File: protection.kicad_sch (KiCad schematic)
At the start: 30 parts, among them J10 10x2.54mm, J5 10x2.54mm, J6 10x2.54mm, J7 10x2.54mm, J8 10x2.54mm, J9 10x2.54mm, K19 TQ2-5, U6 TXS0108EPW, U7 TXS0108EPW, U8 TXS0108EPW

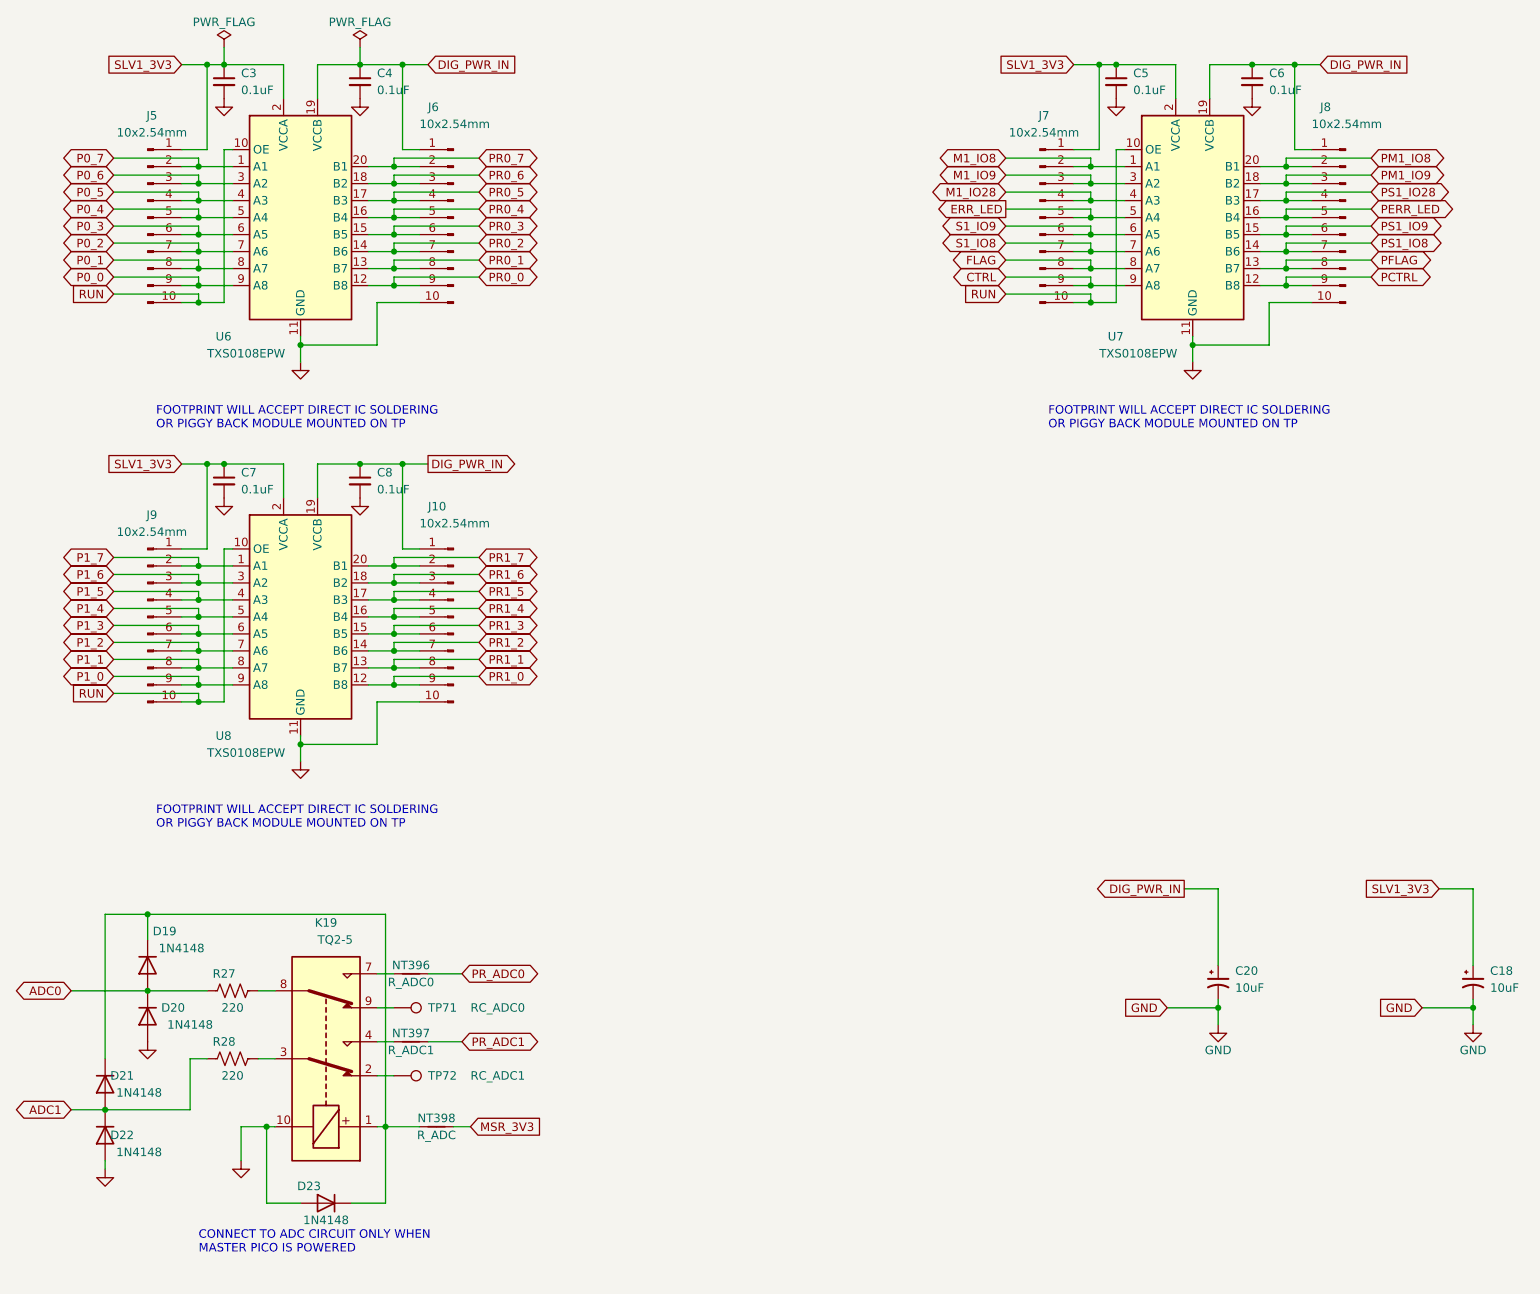
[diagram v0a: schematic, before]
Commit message: update
Correction of small error
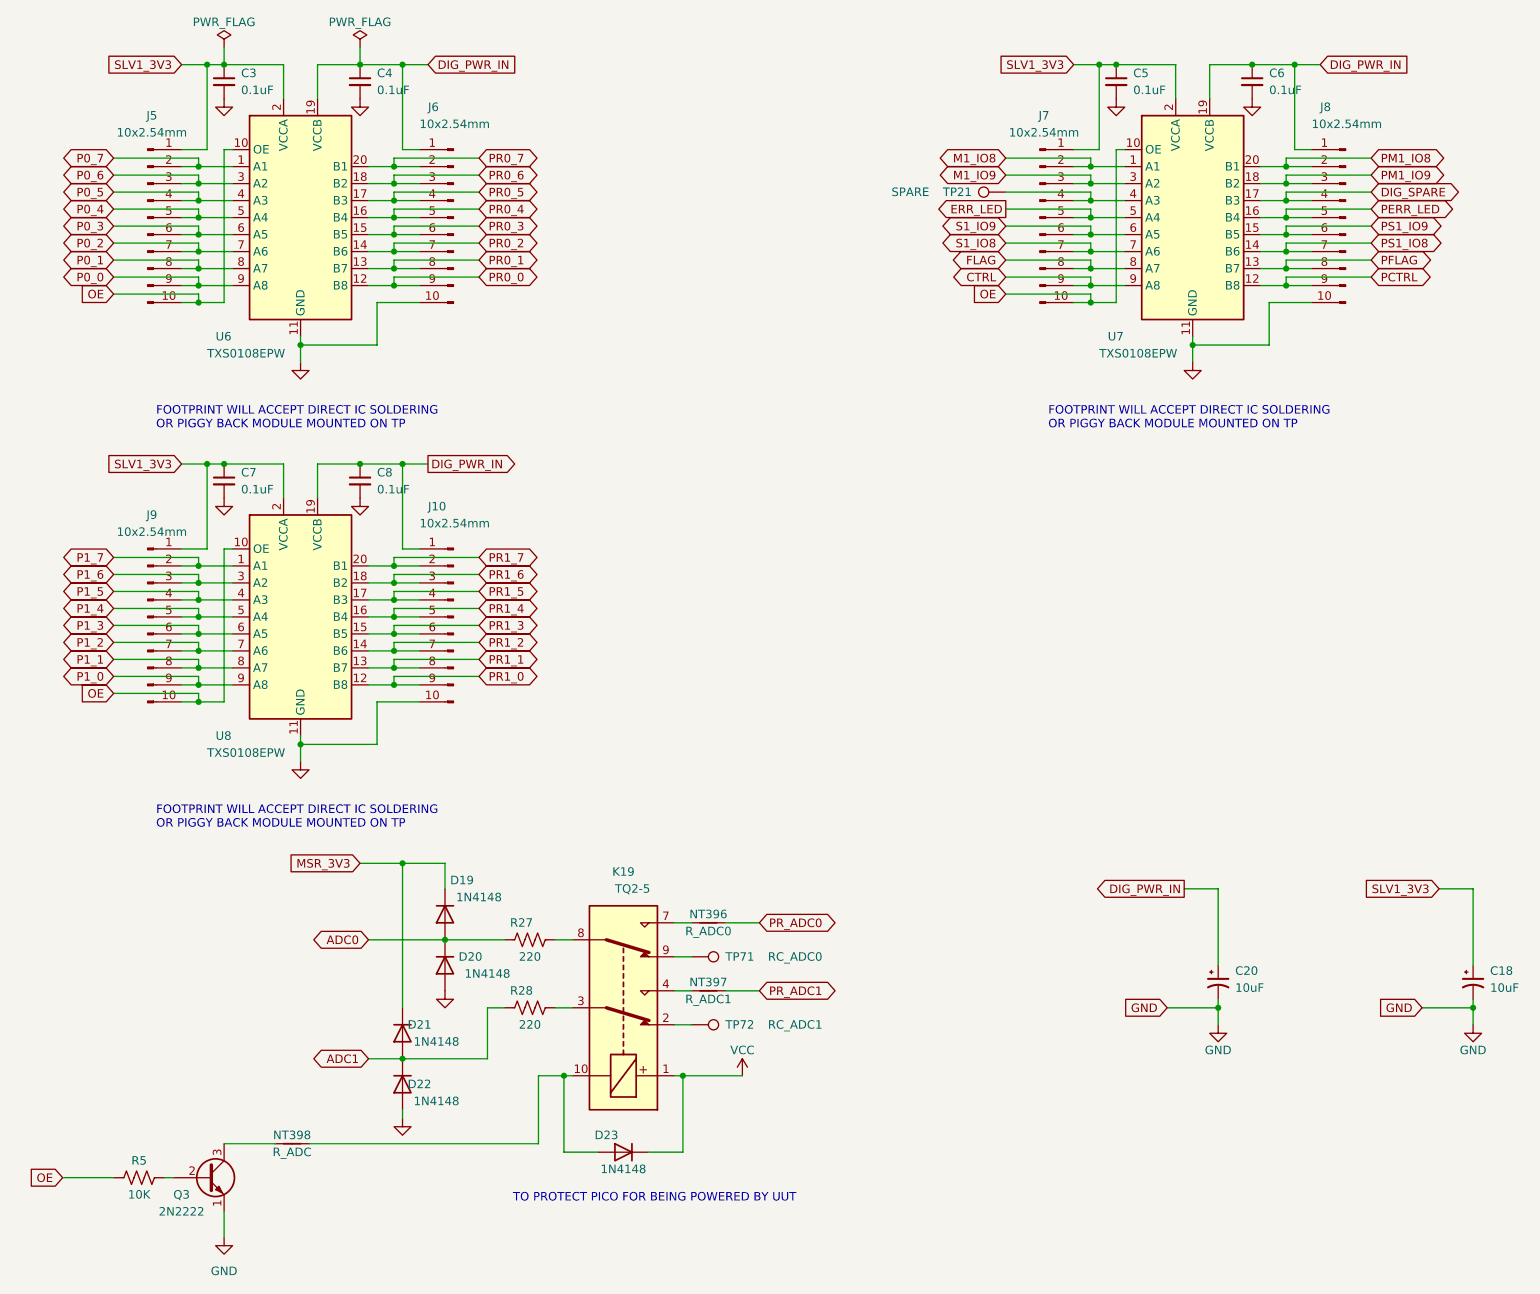
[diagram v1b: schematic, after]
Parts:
- added Q3: 2N2222, Package_TO_SOT_THT:TO-92_Inline, symbol Transistor_BJT:2N3904
- added R5: 10K, Resistor_THT:R_Axial_DIN0207_L6.3mm_D2.5mm_P10.16mm_Horizontal, symbol Device:R_US
- added TP21: SPARE, TestPoint:TestPoint_THTPad_D1.5mm_Drill0.7mm, symbol Connector:TestPoint
- R27, R28: footprint Resistor_THT:R_Axial_DIN0309_L9.0mm_D3.2mm_P12.70mm_Horizontal -> Resistor_THT:R_Axial_DIN0207_L6.3mm_D2.5mm_P10.16mm_Horizontal
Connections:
- net GND: now also Q3.1 (E); no longer D23.2 (A), K19.10
- net MSR_3V3: now also D19.1 (K), D21.1 (K); no longer NT398.1
- net M1_IO28: no longer names the net of J7.4 (Pin_4), U7.4 (A3)
- net M1_IO28: now also TP21.1
- net PS1_IO28 renamed DIG_SPARE
- net RUN renamed OE
- net OE: now also R5.2
- new net: D23.2 (A), K19.10, NT398.1
- new net: Q3.2 (B), R5.1
- new net: NT398.2, Q3.3 (C)
- new net VCC: D23.1 (K), K19.1
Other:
- note added: "TO PROTECT PICO FOR BEING POWERED BY UUT"
- note removed: "CONNECT TO ADC CIRCUIT ONLY WHEN MASTER PICO IS POWERED"
- moved on the sheet: D19, D20, D21, D22, D23, K19, NT396, NT397, R27, R28, TP71, TP72
